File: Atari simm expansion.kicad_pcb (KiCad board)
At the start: 2 copper layers, 112.8 x 55.8 mm, 30 parts, among them J1 4464_A, J10 PB0..7, J11 RAS_sel, J2 4464_B, J3 4464_A, J4 4464_B, J5 SMMU_A, J6 SMMU_B, J7 MMU_A, J8 MMU_A, J9 Mem_On_Off, U1 SIMM_exp_GAL, U10 DRAM_1MB_4bit, U13 74LS04, U2 74LS175, U3 MMU, U4 74LS157, U9 DRAM_1MB_4bit

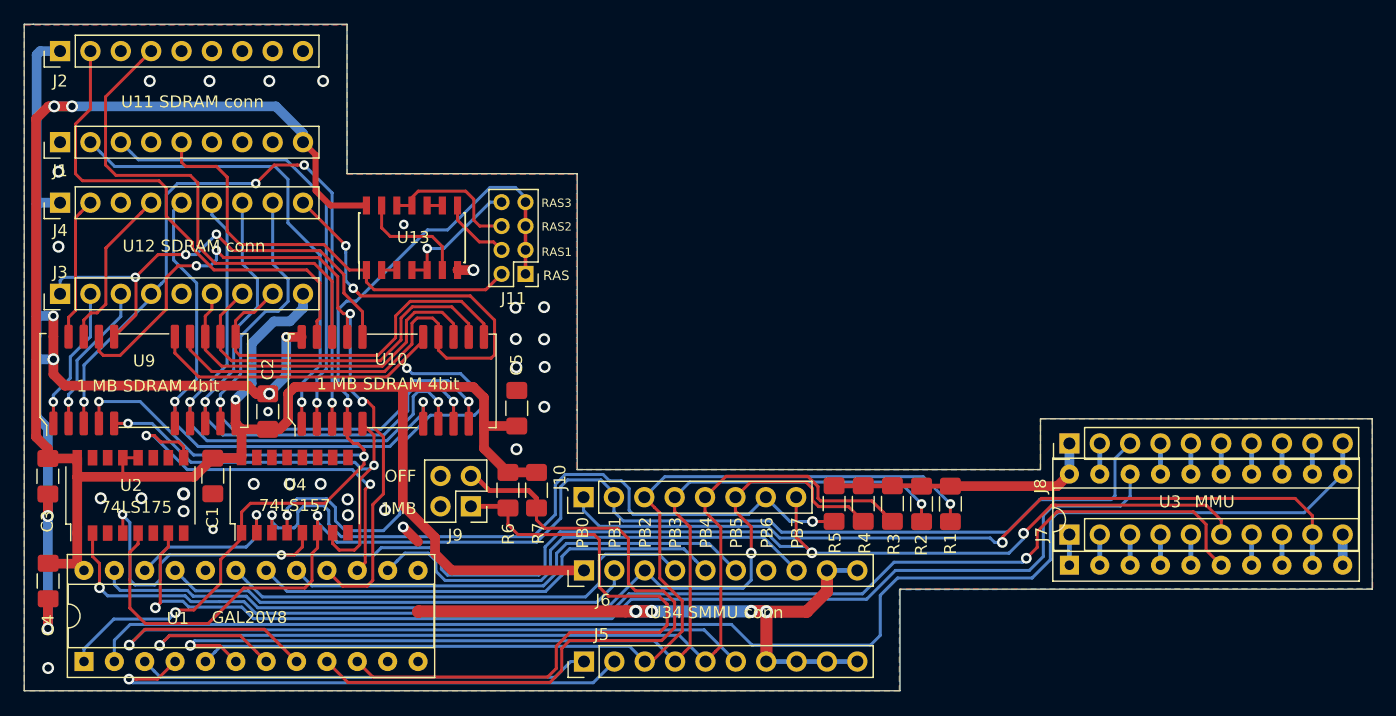
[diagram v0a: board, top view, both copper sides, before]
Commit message: Tracking
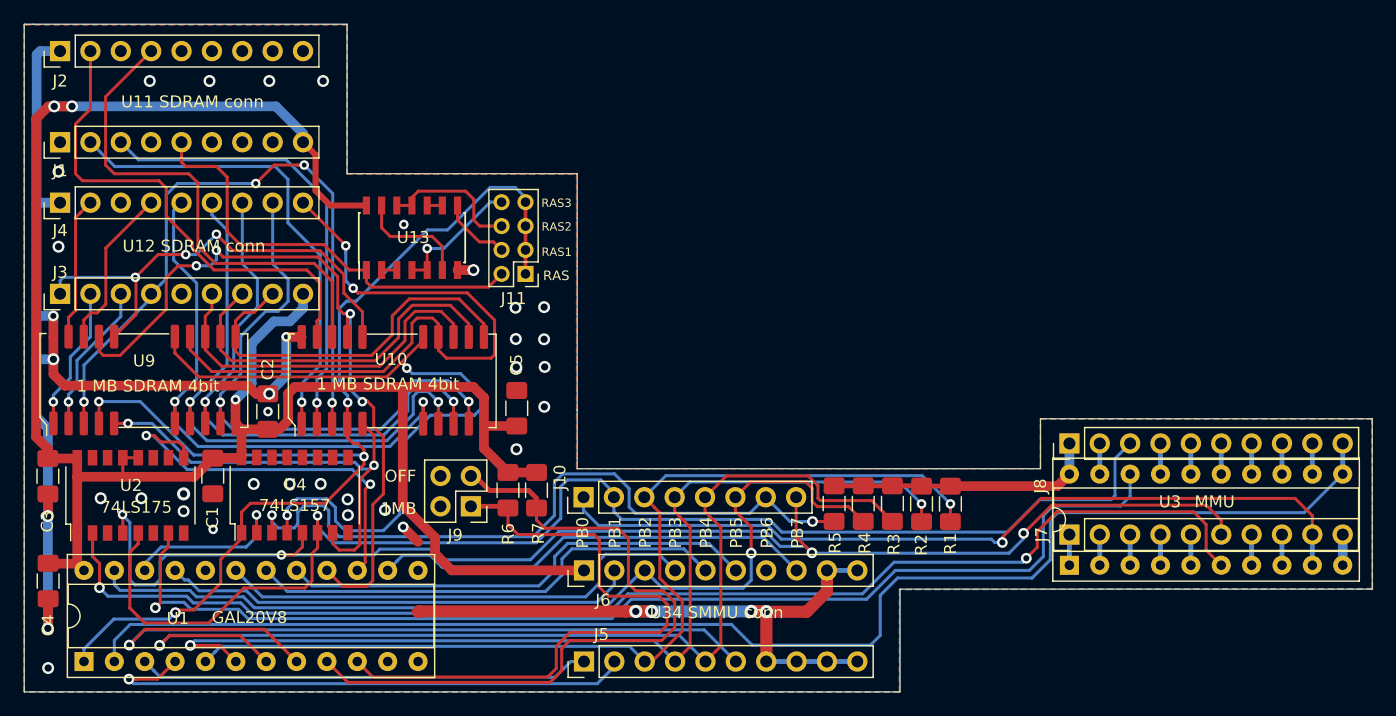
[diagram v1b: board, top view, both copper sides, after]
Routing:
- net HALT: track 39.9 -> 37.3 mm
- net PB7: track 117.6 -> 115.1 mm
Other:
- outline, holes or cut-outs redrawn
